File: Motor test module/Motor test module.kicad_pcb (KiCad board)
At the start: 2 copper layers, 103.1 x 103.1 mm, 55 parts, among them J1 Conn_02x04_Counter_Clockwise, J2 Conn_02x04_Counter_Clockwise, J3 Conn_02x04_Counter_Clockwise, J4 Conn_02x04_Counter_Clockwise, J5 Conn_02x04_Counter_Clockwise, J6 Conn_02x04_Counter_Clockwise, J7 Conn_01x05_Male, J8 Screw_Terminal_01x02, SW1 SW_Push, U1 TPS63060, U10 ATA6560,1, U2 AP1017AEN, U3 AP1017AEN, U4 AP1017AEN, U5 AP1017AEN, U6 AP1017AEN, U7 AP1017AEN, U8 ATmega2560-16AU, U9 MCP2515-EST, Y1 16MHz, Y2 16MHz

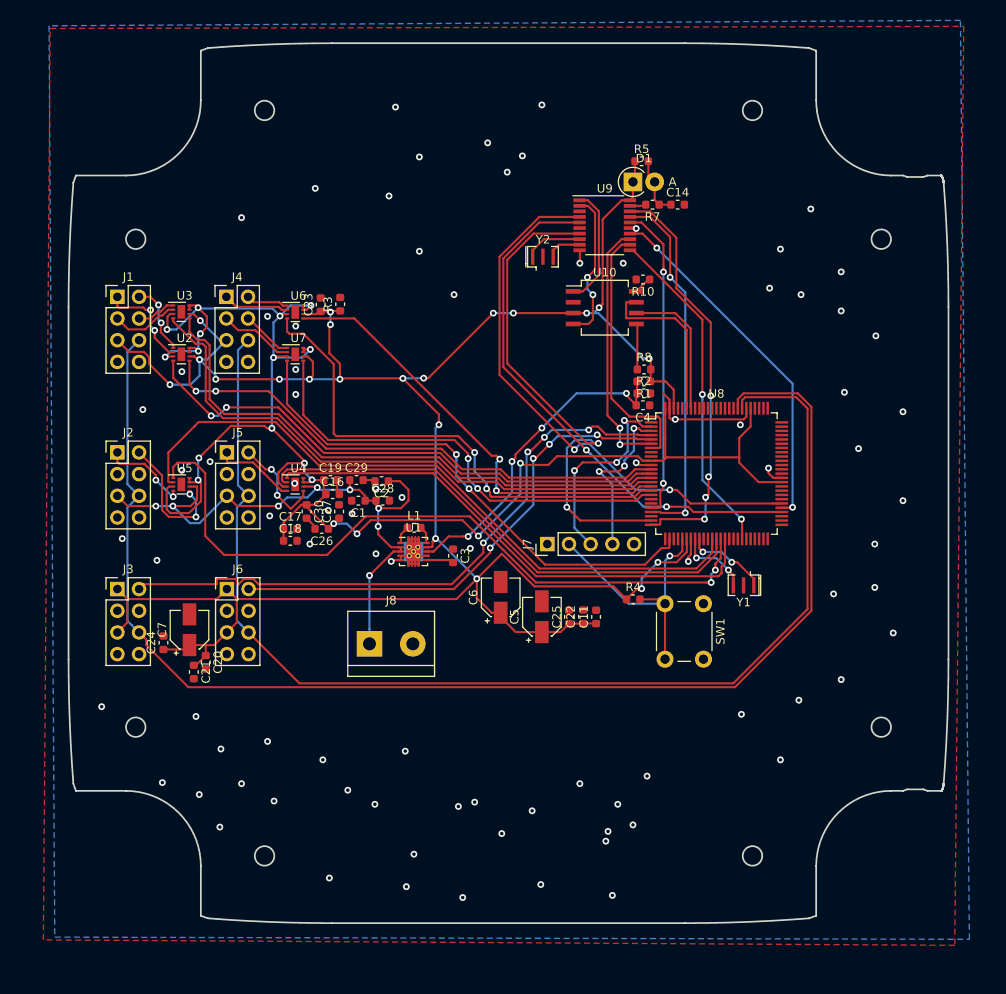
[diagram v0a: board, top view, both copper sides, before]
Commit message: Fourth draft of layout
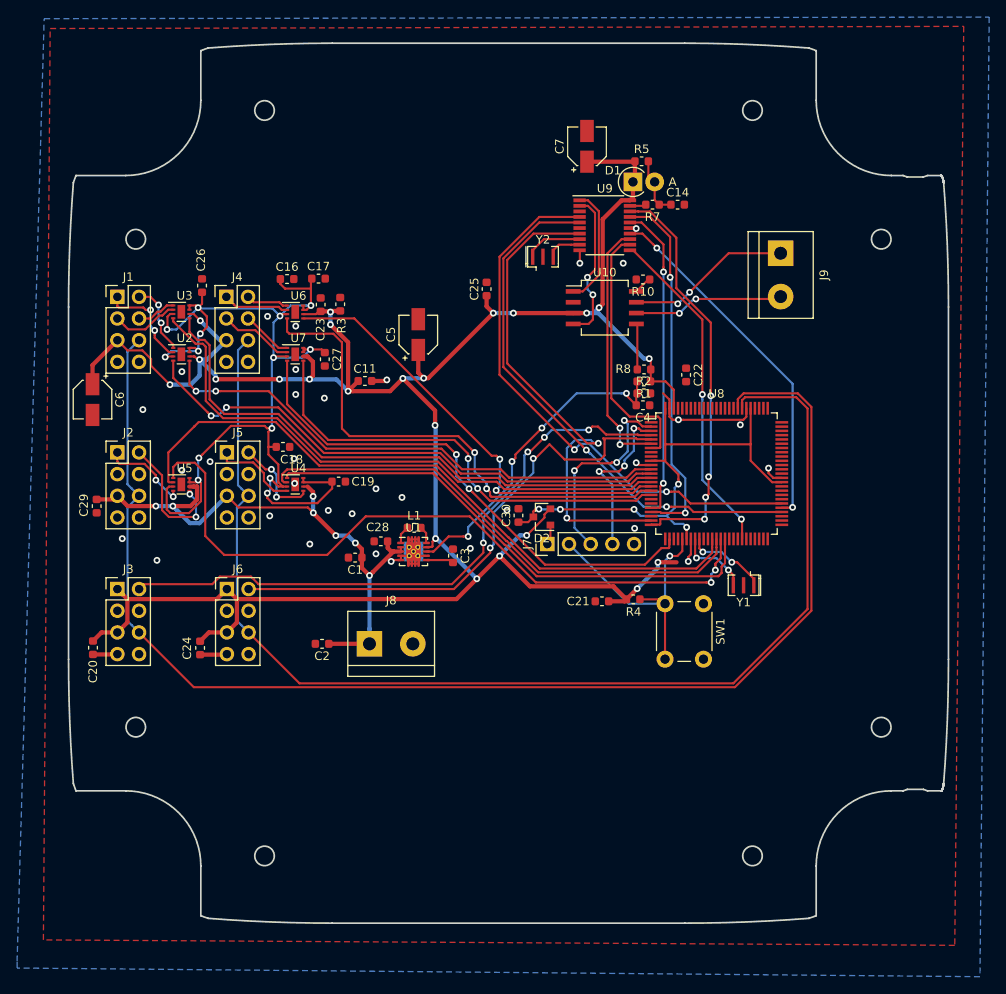
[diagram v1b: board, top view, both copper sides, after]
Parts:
- added D2: D_x2_KCom_AAK, Package_TO_SOT_SMD:SOT-23, F.Cu at (138.4, 106.6)
- added J9: Screw_Terminal_01x02, TerminalBlock:TerminalBlock_bornier-2_P5.08mm, F.Cu at (166.4, 75.7)
- moved C7 73.3 mm to (143.7, 63.1)
- moved C6 53.1 mm to (85.8, 92.8), turned to 270 degrees
- moved C21 48.5 mm to (145.5, 116.4), turned to 180 degrees
- moved C25 39.6 mm to (132.0, 79.9)
- moved C11 38.7 mm to (117.7, 90.6), turned to 0 degrees
- moved C5 36.1 mm to (124.0, 85.2)
- moved C26 31.8 mm to (98.6, 79.5), turned to 90 degrees
- moved C22 30.8 mm to (155.3, 89.9), turned to 270 degrees
- moved C29 30.6 mm to (86.3, 105.3), turned to 270 degrees
- moved C17 29.5 mm to (112.3, 78.6)
- moved C16 25.8 mm to (108.6, 78.7)
- moved C30 24.8 mm to (135.7, 106.4), turned to 90 degrees
- moved C2 20.3 mm to (112.7, 121.4)
- moved C27 17.9 mm to (113.0, 88.1), turned to 270 degrees
- moved C20 13.3 mm to (85.9, 121.9)
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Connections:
- C30 pad 1: +3V3 -> VCC
- U8 pad 10: +5V -> VCC
- U8 pad 100: +5V -> VCC
- U8 pad 31: +5V -> VCC
- U8 pad 61: +5V -> VCC
- U8 pad 80: +5V -> VCC
- U8 pad 94: CANL -> Net-(U8-Pad94)
- U8 pad 95: CANH -> Net-(U8-Pad95)
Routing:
- net VCC: track 0.00 -> 59.3 mm, vias 0 -> 5
- net +3V3: track 162.7 -> 122.4 mm, vias 18 -> 14
- net +5V: track 304.2 -> 281.6 mm, vias 21 -> 23
- net +12V: track 72.4 -> 69.1 mm, vias 8 -> 7
- net GNDREF: track 35.4 -> 38.4 mm, vias 87 -> 33
- net Servo2: track 58.4 -> 60.9 mm, vias 4 -> 2
- net Net-(D2-Pad1): track 0.00 -> 2.38 mm
- net CANL: track 16.4 -> 17.7 mm, vias 0 -> 2
- net M2A-C: track 59.2 -> 60.3 mm
- net M2-: track 11.8 -> 10.6 mm
- net Servo1: track 73.8 -> 72.9 mm
- net TX2: track 58.1 -> 58.9 mm
- net M2+: track 9.56 -> 10.1 mm
- net CANH: track 19.8 -> 19.4 mm, vias 0 -> 2
